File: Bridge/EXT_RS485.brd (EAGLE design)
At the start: 22.5 x 72 mm, 8 parts, among them IC1 SN65HVD72D, X1 V1, X2 GND, X3 V2

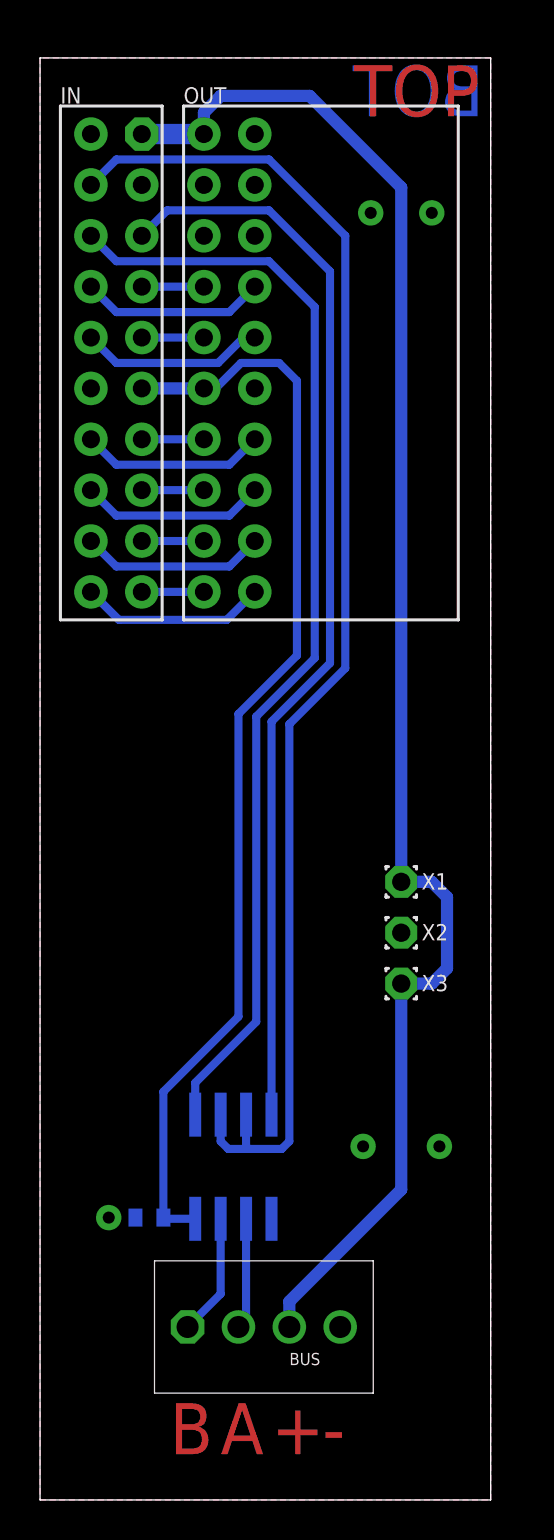
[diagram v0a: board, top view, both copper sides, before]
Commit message: Minor Changes
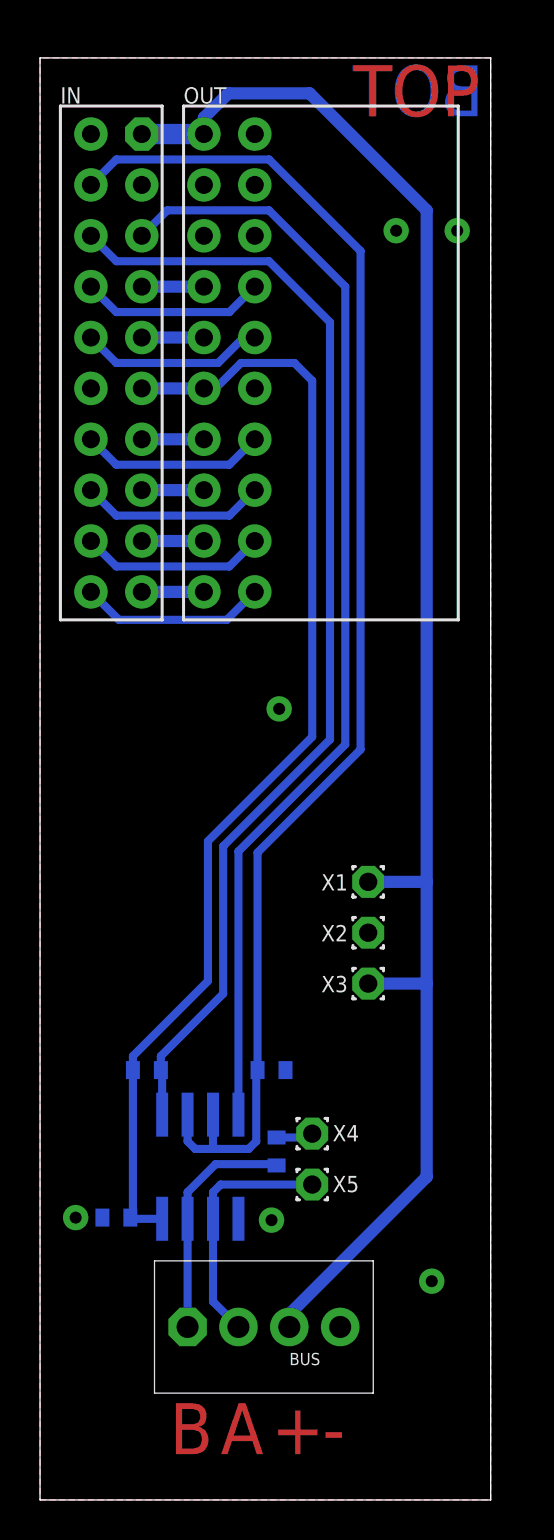
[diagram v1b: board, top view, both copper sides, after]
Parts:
- added R1, R3: 10k, RCL:0603
- added R2: 120R, RCL:0603
- added X4, X5: TERM, Conn:T1.6/0.9
- moved C1 1.65 mm to (3.81, 14.1)
- moved IC1 1.65 mm to (8.00, 16.6)
- moved X1 1.65 mm to (16.4, 30.9), turned to 180 degrees
- moved X2 1.65 mm to (16.4, 28.3), turned to 180 degrees
- moved X3 1.65 mm to (16.4, 25.8), turned to 180 degrees
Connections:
- new net N$13: R2.1, X4.1
- net +3V3: now also R3.2
- net DE: now also R1.2
- net GND: now also R1.1
- net N$11: now also R2.2
- net N$12: now also X5.1
- net RX: now also R3.1
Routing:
- net N$12: track 5.56 -> 12.4 mm
- net N$11: track 6.08 -> 11.8 mm
- net VIN: track 79.2 -> 82.4 mm
- net N$13: track 0.00 -> 1.86 mm
- net +3V3: track 54.9 -> 56.7 mm
- net RX: track 55.4 -> 56.8 mm
- net TX: track 54.5 -> 55.8 mm
- net DE: track 68.0 -> 69.3 mm
